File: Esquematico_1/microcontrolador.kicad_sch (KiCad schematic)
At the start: 31 parts, among them U2 STM32F405RGTx, Y1 Crystal

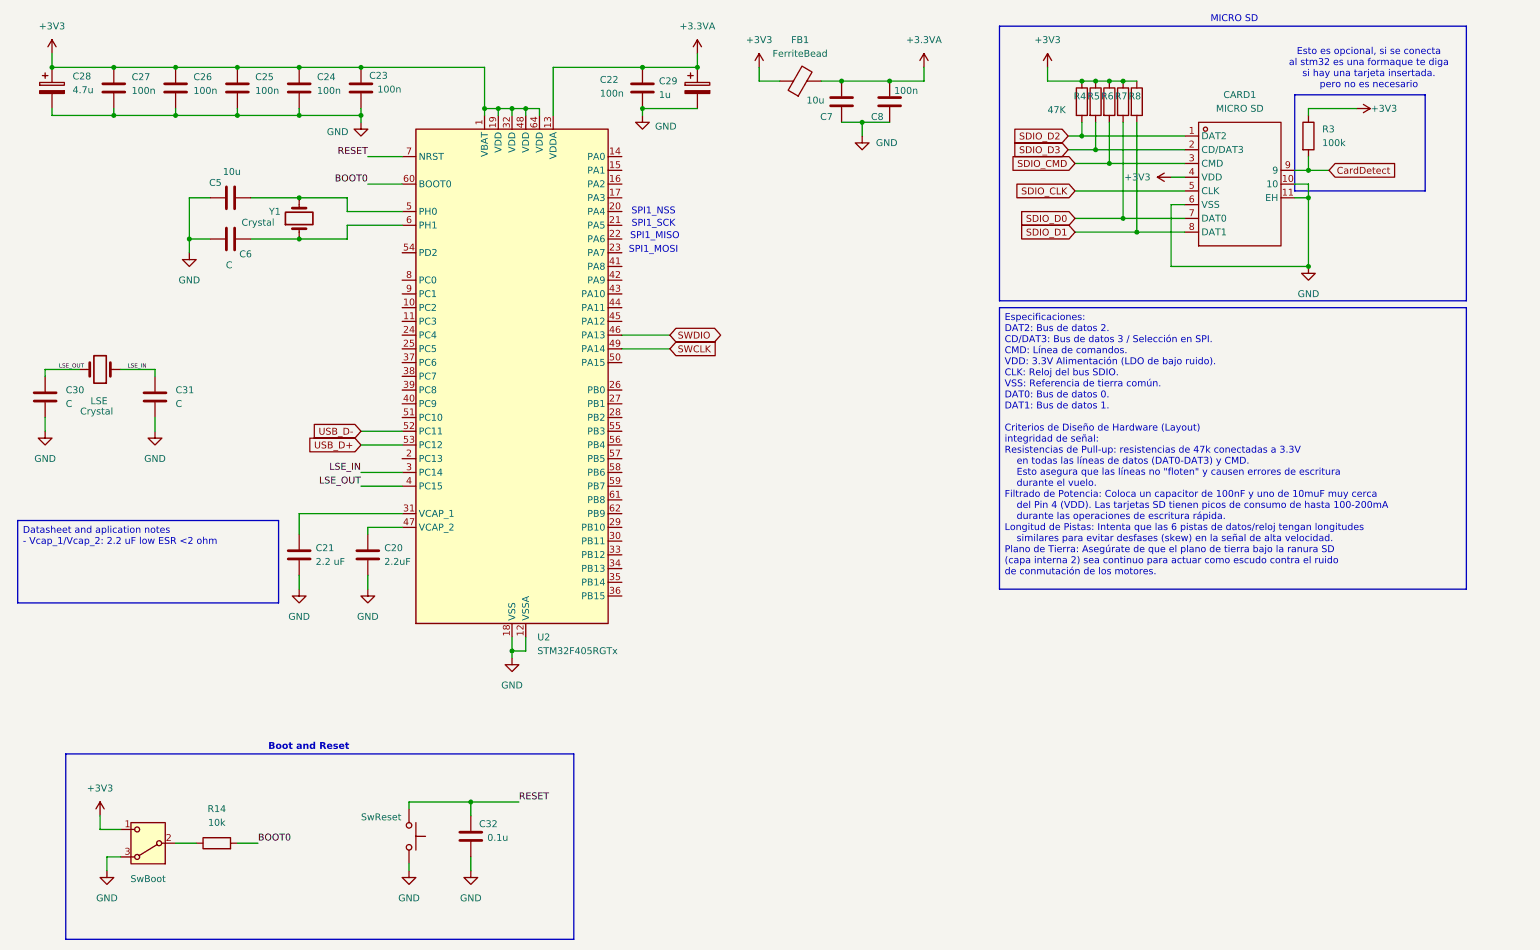
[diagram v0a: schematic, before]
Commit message: Cristales y arreglo de los simbolos que no estaban en referencia
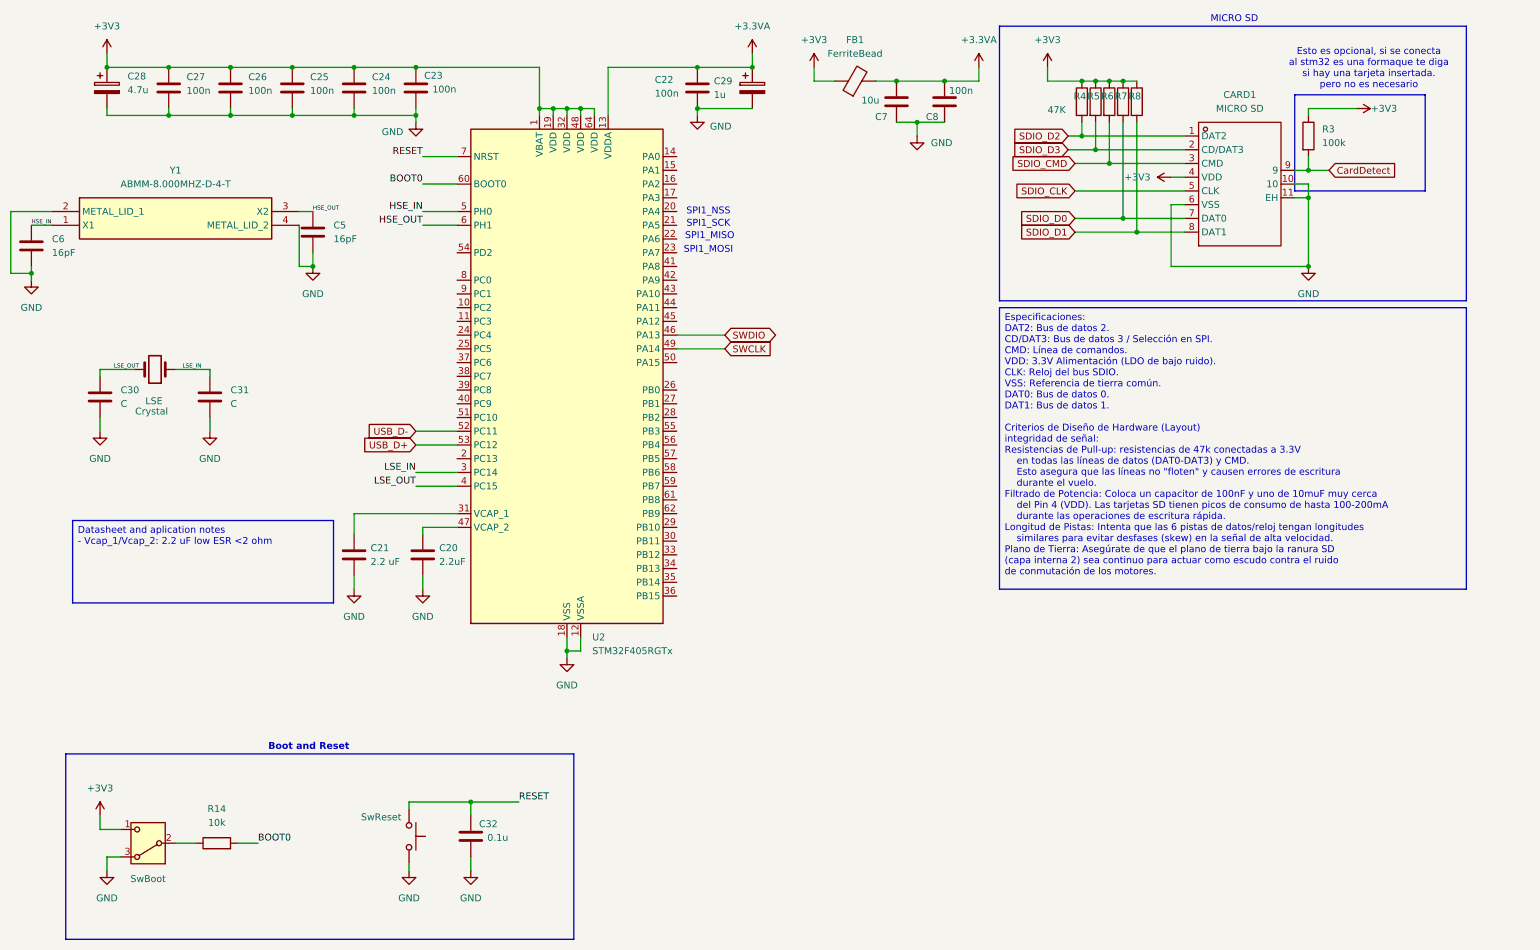
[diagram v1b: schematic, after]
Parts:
- removed Y1: Crystal, symbol Device:Crystal
- added Y1: ABMM-8.000MHZ-D-4-T, ABMM25000MHZB2T, symbol ABMM-8_000MHZ-D-4-T:ABMM-8.000MHZ-D-4-T
- C5: value 10u -> 16pF
- C6: value C -> 16pF
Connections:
- net GND: now also C5.2, Y1.2 (METAL_LID_1), Y1.4 (METAL_LID_2); no longer C5.1
- net HSE_IN: now reaches U2.5 (PH0)
- net HSE_IN: now also C6.1, Y1.1 (X1); no longer C5.2
- net HSE_OUT: now reaches U2.6 (PH1)
- net HSE_OUT: now also C5.1, Y1.3 (X2); no longer C6.1
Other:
- moved on the sheet: C20, C21, C22, C23, C24, C25, C26, C27, C28, C29, C30, C31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
